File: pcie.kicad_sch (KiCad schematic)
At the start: 10 parts, among them U1 MPFS250T-FCVG484, U17 DSC557-0343FI1

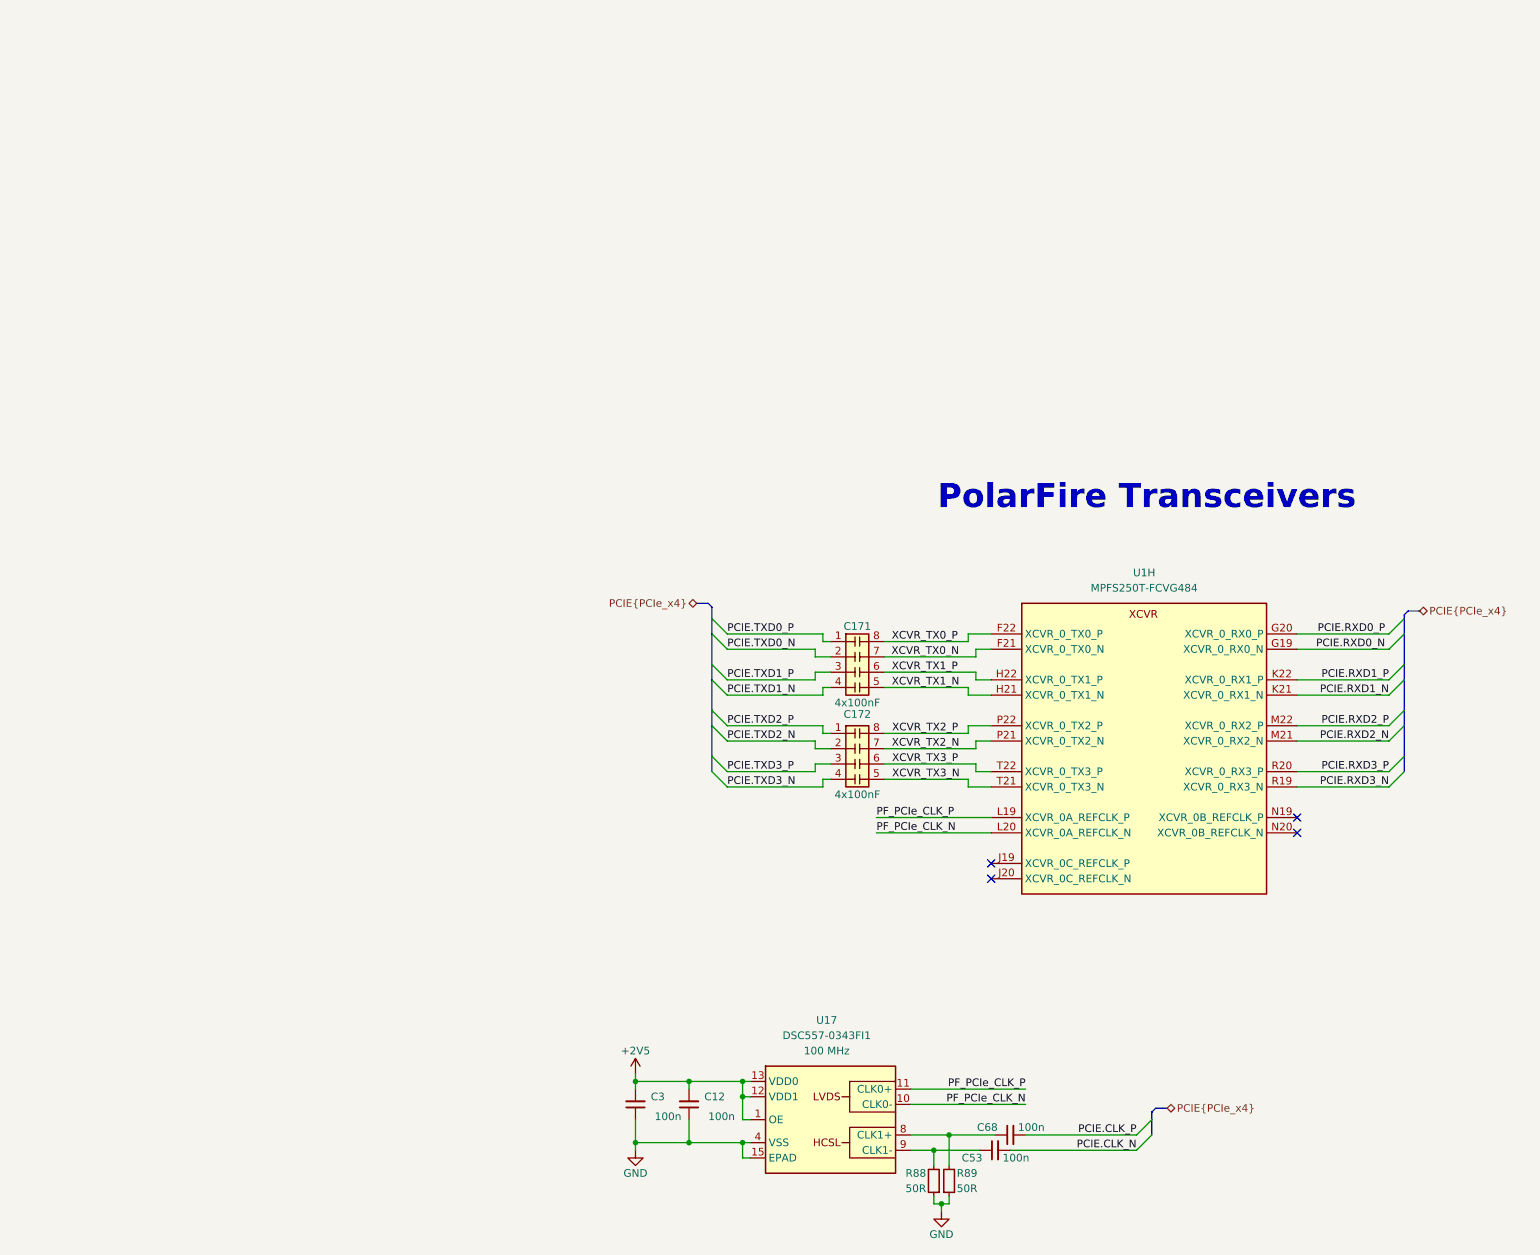
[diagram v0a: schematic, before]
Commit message: [#57422] Finishing touches
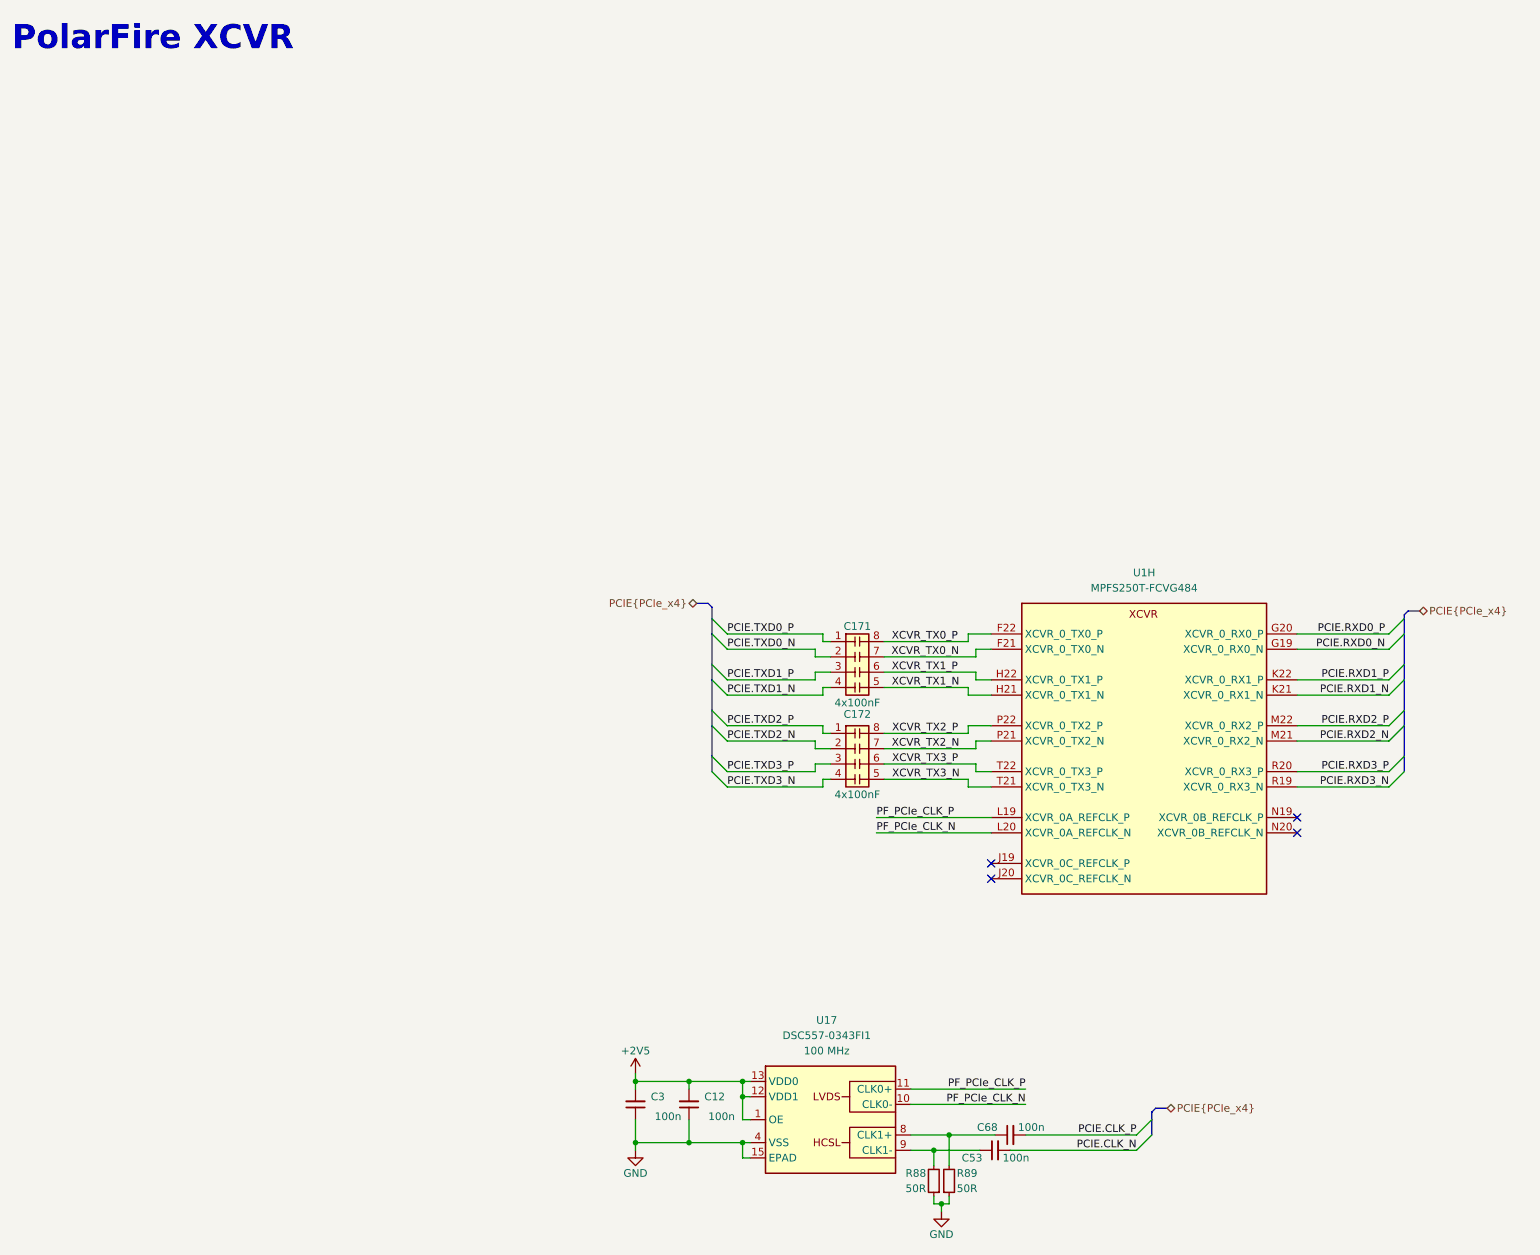
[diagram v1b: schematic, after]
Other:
- note added: "PolarFire XCVR"
- note removed: "PolarFire Transceivers"
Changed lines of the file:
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@@
   (title_block
     (title "PolarFire SoM")
-    (date "2024-04-03")
+    (date "2024-04-08")
     (rev "1.0.0")
     (company "Antmicro Ltd")
@@
     )
   )
-  (text "PolarFire Transceivers" (at 168.91 97.79 0)
+  (text "PolarFire XCVR" (at 15.24 21.59 0)
     (effects (font (size 4 4) (thickness 0.8) bold) (justify left bottom))
   )
